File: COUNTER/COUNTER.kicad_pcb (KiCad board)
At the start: 2 copper layers, 76.1 x 64.6 mm, 28 parts, among them J1 Conn_01x08, J10 Conn_01x04, J2 Conn_01x04, J3 Conn_01x08, U46 74LS161, U47 74LS245, U48 74LS161

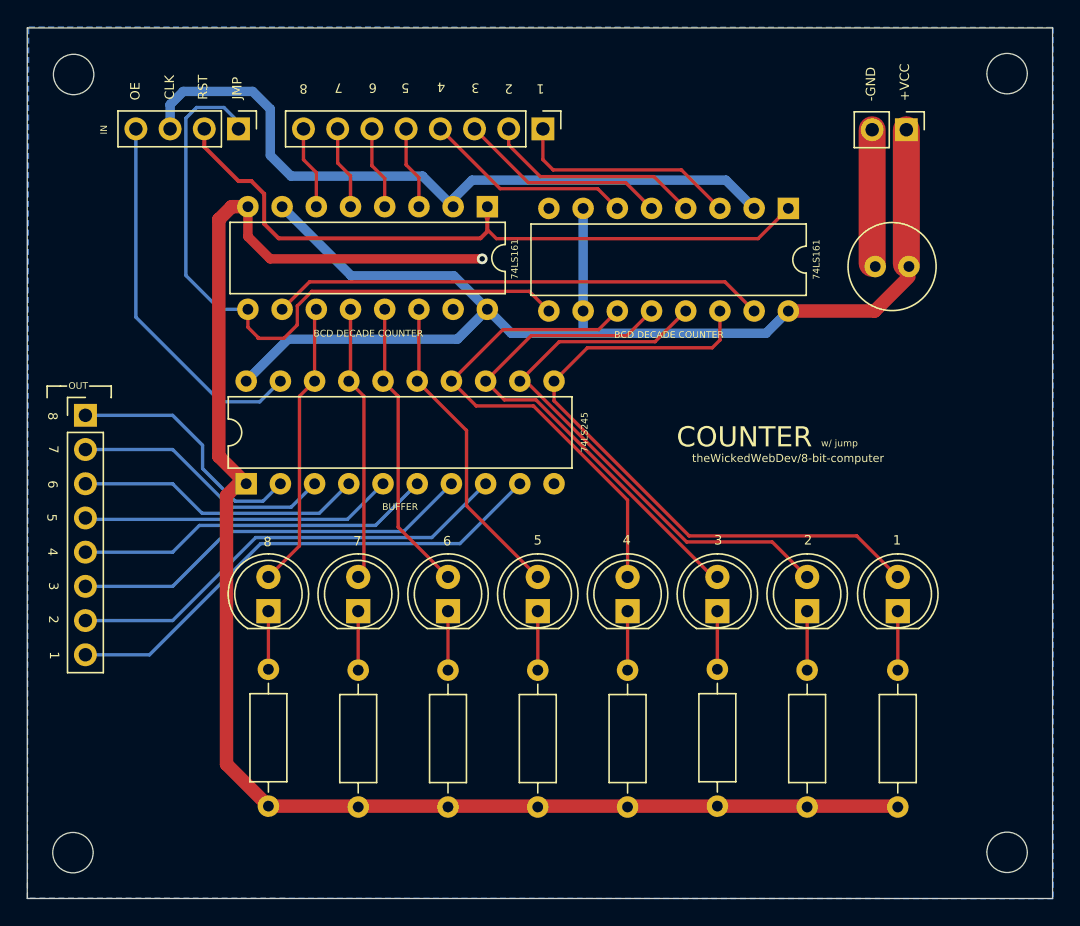
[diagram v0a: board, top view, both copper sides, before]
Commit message: Updating components
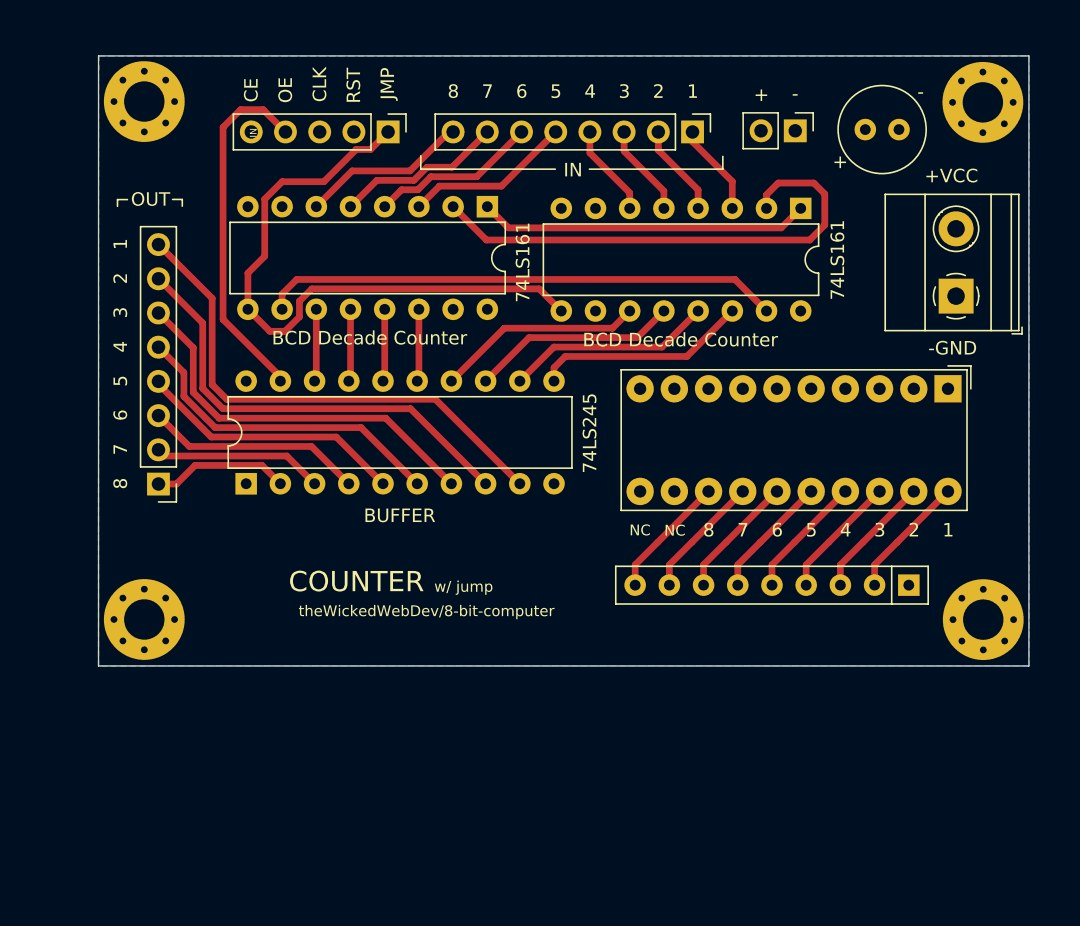
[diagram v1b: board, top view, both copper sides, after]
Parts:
- removed D44, D45, D46, D47, D48, D49, D50, D51: LED, LED_THT:LED_D5.0mm
- removed R11, R12, R13, R14, R15, R16, R17, R18: R_US, Resistor_THT:R_Axial_DIN0207_L6.3mm_D2.5mm_P10.16mm_Horizontal
- removed the REF** at (74.9, 90.3)
- removed the REF** at (74.9, 32.5)
- removed the REF** at (144.3, 90.3)
- removed the REF** at (144.3, 32.5)
- added BAR1: HDSP-4830_2, Display:HDSP-4830, F.Cu at (139.9, 55.9)
- added J1: Screw_Terminal_01x02, TerminalBlock_Phoenix:TerminalBlock_Phoenix_MKDS-1,5-2_1x02_P5.00mm_Horizontal, F.Cu at (140.5, 49.0)
- added REF**: MountingHole_3mm_Pad_Via, MountingHole:MountingHole_3mm_Pad_Via, F.Cu at (142.5, 73.0)
- added REF**: MountingHole_3mm_Pad_Via, MountingHole:MountingHole_3mm_Pad_Via, F.Cu at (80.2, 73.0)
- added REF**: MountingHole_3mm_Pad_Via, MountingHole:MountingHole_3mm_Pad_Via, F.Cu at (142.5, 34.6)
- added REF**: MountingHole_3mm_Pad_Via, MountingHole:MountingHole_3mm_Pad_Via, F.Cu at (80.2, 34.5)
- added RN1: R_Network08, Resistor_THT:R_Array_SIP9, F.Cu at (137.0, 70.5)
- J22: renamed from J2; value Conn_01x04 -> Conn_01x05; footprint Connector_PinHeader_2.54mm:PinHeader_1x04_P2.54mm_Vertical -> Connector_PinHeader_2.54mm:PinHeader_1x05_P2.54mm_Vertical
- moved J22 11.1 mm to (98.3, 36.8)
- moved J23 11.1 mm to (120.9, 36.8)
- moved C10 10.7 mm to (133.7, 36.6), turned to 0 degrees
- moved J10 8.25 mm to (128.5, 36.7)
- moved J24 7.45 mm to (81.2, 62.9), turned to 180 degrees
- moved U14 0.92 mm to (128.9, 42.5)
- renumbered C8 to C10, J3 to J23, J1 to J24, U46 to U12, U48 to U14
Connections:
- net /CLOCK renamed CLOCK
- net /D1 renamed D1
- net /D2 renamed D2
- net /D3 renamed D3
- net /D4 renamed D4
- net /D5 renamed D5
- net /D6 renamed D6
- net /D7 renamed D7
- net /D8 renamed D8
- net /JUMP renamed JUMP
- net /OE renamed OE
- net /RESET renamed RESET
- net /Y1 renamed Y1
- net /Y2 renamed Y2
- net /Y3 renamed Y3
- net /Y4 renamed Y4
- net /Y5 renamed Y5
- net /Y6 renamed Y6
- net /Y7 renamed Y7
- net /Y8 renamed Y8
- J10 pad 1: VCC -> GND
- J10 pad 2: GND -> VCC
- U14 pad 10: VCC -> CE
- U14 pad 7: VCC -> CE
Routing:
- net GND: track 126.5 -> 0.00 mm, vias 1 -> 0
- net VCC: track 92.6 -> 0.00 mm
- net CE: track 0.00 -> 37.6 mm
- net RESET: track 55.7 -> 37.3 mm
- net Net-(BAR1-Pad7): track 20.6 -> 37.0 mm
- net Net-(BAR1-Pad8): track 21.3 -> 37.0 mm
- net Net-(BAR1-Pad6): track 21.9 -> 37.0 mm
- net Net-(BAR1-Pad1): track 48.1 -> 34.4 mm
- net Net-(BAR1-Pad5): track 23.6 -> 37.0 mm
- net D1: track 16.9 -> 6.90 mm
- net D2: track 16.3 -> 6.90 mm
- net Net-(BAR1-Pad19): track 0.00 -> 9.22 mm
- net Net-(BAR1-Pad18): track 0.00 -> 9.22 mm
- net Net-(BAR1-Pad16): track 0.00 -> 9.22 mm
- net Net-(BAR1-Pad14): track 0.00 -> 9.22 mm
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- added copper zone on In2.Cu, net VCC
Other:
- board size 76.1 x 64.6 mm -> 69.1 x 45.3 mm
- copper layers 2 -> 4
- board text added: "+"
- board text added: "-"
- board text added: "BCD Decade Counter"
- board text added: "CE"
- board text added: "NC"
- board text removed: "BCD DECADE COUNTER"
